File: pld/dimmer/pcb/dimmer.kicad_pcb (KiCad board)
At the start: 2 copper layers, 74.9 x 41.4 mm, 25 parts, among them J1 MCU, J2 AC/Load, J3 H2, J4 H1, Q1 BTA20, SW1 PWM, U1 GAL16V8, U2 4N35, U3 LM555, U4 MOC3052M

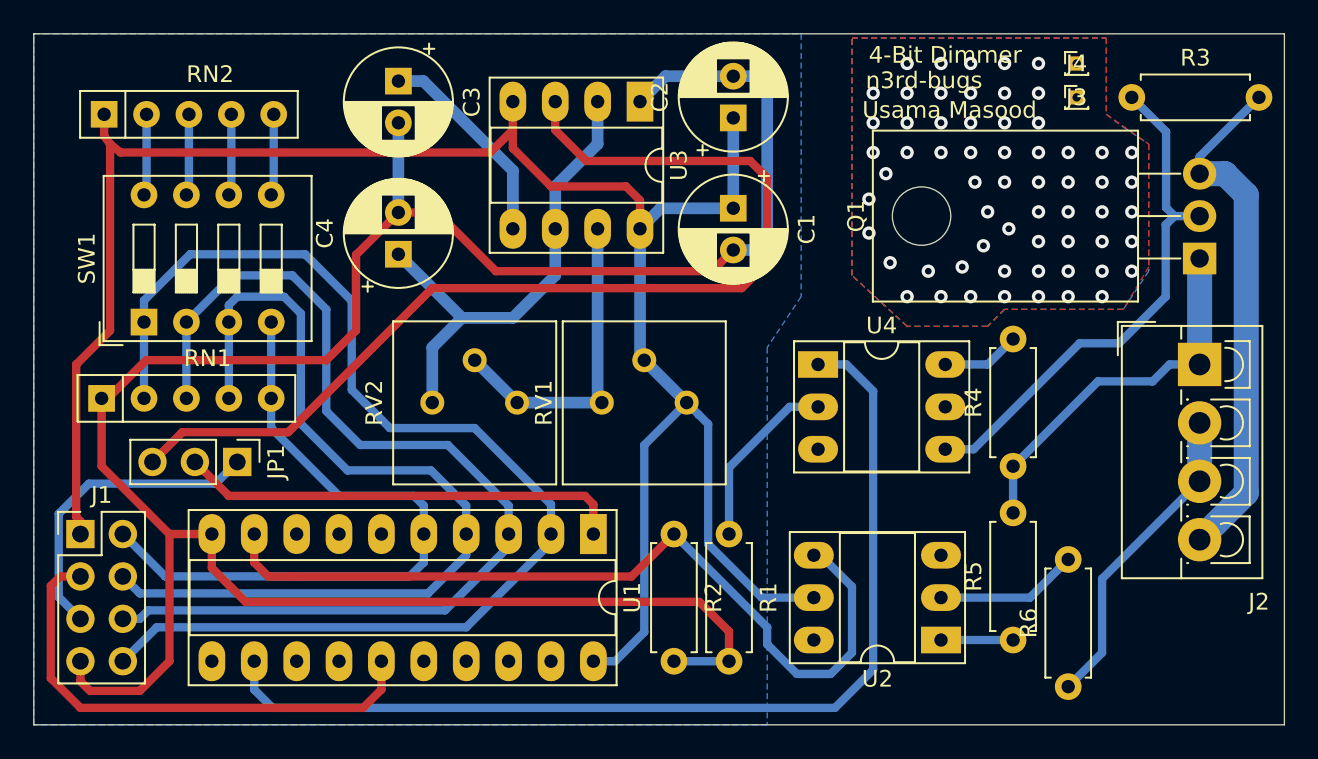
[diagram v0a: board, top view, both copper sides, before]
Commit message: Updated PCB with latest changes.
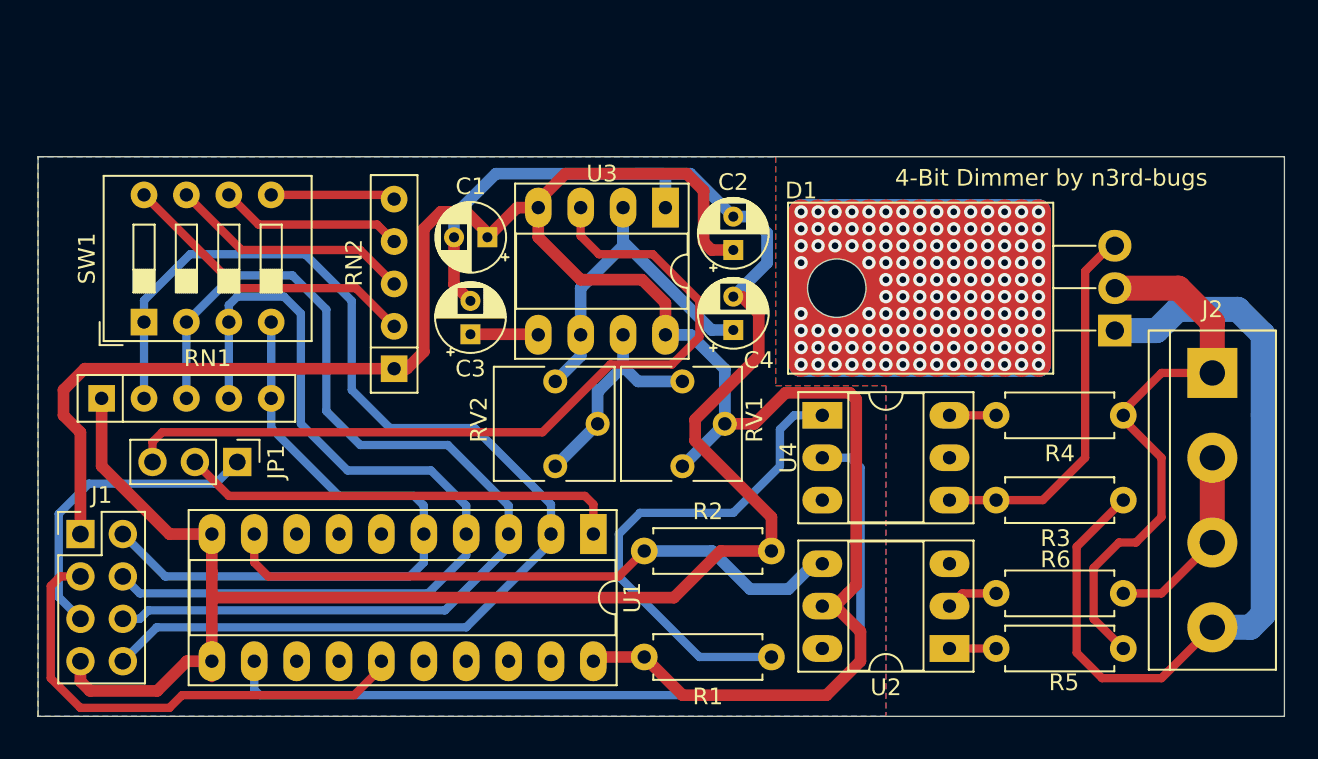
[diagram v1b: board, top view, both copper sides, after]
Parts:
- removed J3: H2, Connector_PinHeader_1.00mm:PinHeader_1x01_P1.00mm_Vertical
- removed J4: H1, Connector_PinHeader_1.00mm:PinHeader_1x01_P1.00mm_Vertical
- removed Q1: BTA20, Package_TO_SOT_THT:TO-220-3_Horizontal_TabDown
- added D1: BTA20, Package_TO_SOT_THT:TO-220-3_Horizontal_TabDown, F.Cu at (188.2, 79.0)
- C1, C2, C3, C4: footprint Capacitor_THT:CP_Radial_D6.3mm_P2.50mm -> Capacitor_THT:CP_Radial_D4.0mm_P2.00mm
- J2: footprint TerminalBlock_4Ucon:TerminalBlock_4Ucon_1x04_P3.50mm_Vertical -> TerminalBlock:TerminalBlock_bornier-4_P5.08mm
- R5, R6: value 20k -> 100k
- RV1, RV2: footprint Potentiometer_THT:Potentiometer_Bourns_3386P_Vertical -> Potentiometer_THT:Potentiometer_Vishay_T73YP_Vertical
- moved R3 25.5 mm to (181.1, 89.2)
- moved RN2 23.1 mm to (145.0, 81.3), turned to 90 degrees
- moved C4 20.6 mm to (165.4, 79.0)
- moved C3 15.8 mm to (149.6, 79.2), turned to 90 degrees
- moved C1 14.8 mm to (150.6, 73.4), turned to 180 degrees
- moved C2 7.91 mm to (165.4, 74.2)
- moved R1 7.79 mm to (167.6, 98.6), turned to 180 degrees
- moved R4 7.27 mm to (188.7, 84.1), turned to 180 degrees
- moved U3 6.53 mm to (161.3, 71.6)
- moved R6 6.49 mm to (188.7, 94.7), turned to 180 degrees
- moved RV2 4.44 mm to (154.7, 87.1), turned to 0 degrees
- moved RV1 3.82 mm to (162.3, 87.1), turned to 0 degrees
- moved U4 3.06 mm to (170.7, 84.1)
- moved R2 2.05 mm to (160.0, 92.2), turned to 0 degrees
- moved R5 1.14 mm to (181.1, 98.0), turned to 0 degrees
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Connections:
- R1 pad 2: GNDD -> +5V
- U1 pad 11: (no net) -> GNDD
- U4 pad 1: TRIG -> Net-(R1-Pad1)
- U4 pad 2: Net-(R1-Pad1) -> TRIG
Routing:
- net (no net): track 0.00 -> 431.1 mm, vias 0 -> 134
- net Net-(D1-Pad1): track 31.2 -> 50.5 mm
- net Net-(R1-Pad1): track 10.8 -> 30.1 mm
- net GNDD: track 139.4 -> 120.5 mm
- net Net-(RN2-Pad2): track 4.89 -> 18.2 mm
- net CLK555: track 62.4 -> 49.2 mm
- net Line: track 50.5 -> 38.3 mm
- net Net-(D1-Pad2): track 22.8 -> 34.4 mm
- net +5V: track 122.8 -> 133.0 mm
- net Net-(RN2-Pad3): track 4.89 -> 14.7 mm
- net Net-(D1-Pad3): track 31.7 -> 22.8 mm
- net Net-(C3-Pad1): track 12.6 -> 4.08 mm
- net TRIG: track 60.8 -> 53.1 mm
- net Net-(J2-Pad2): track 19.1 -> 11.7 mm
- net Net-(C4-Pad1): track 29.3 -> 22.9 mm
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- added copper zone on F.Cu, net +5V
- removed copper zone on B.Cu, net Net-(J3-Pad1)
- removed copper zone on F.Cu, net Net-(J3-Pad1)
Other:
- board size 74.9 x 41.4 mm -> 74.7 x 33.5 mm
- board text added: "4-Bit Dimmer by n3rd-bugs"
- board text removed: "4-Bit Dimmer"
- board text removed: "Usama Masood"
- board text removed: "n3rd-bugs"
